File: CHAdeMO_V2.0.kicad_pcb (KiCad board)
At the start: 4 copper layers, 100 x 107.7 mm, 128 parts, among them IC1 ISO1050DUBR, IC2 ISO1050DUBR, IC3 ATSAM3X8CA-CU, J1 UJ2-BV-1-TH, J2 5810132011, J3 39-28-8020, J4 B2B-PH-K-S(LF)(SN), K1 V23086C1001A403-EV-BLBOX, Q1 IRLML0060TRPBF, Q2 IRLML0060TRPBF, Q3 IRLML0060TRPBF, Q4 IRLML0060TRPBF, Q5 DMP4065SQ-7, U1 M24M02-DRMN6TP, U3 VOM617A-4T, U4 VOM617A-4T, U5 VOM617A-4T, U6 VOM617A-4T, U7 VOM617A-4T, Y1 CRYSTAL 12MHZ, Y2 Crystal 32.768kHz

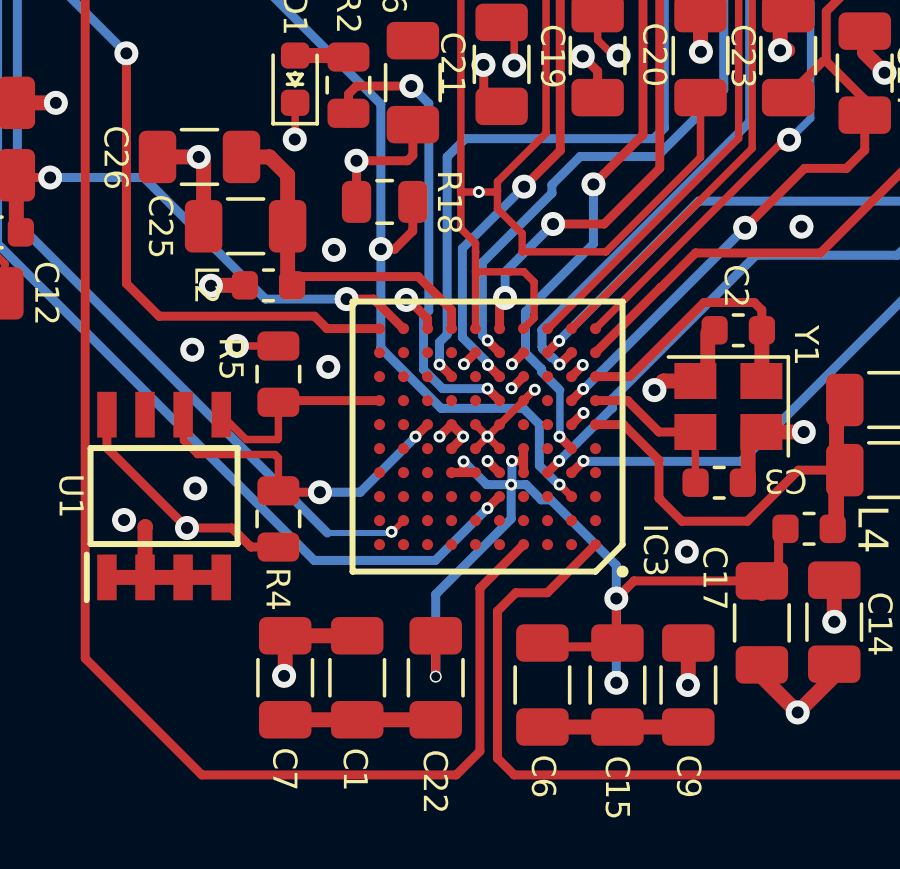
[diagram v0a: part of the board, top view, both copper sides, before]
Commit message: 2.0.3 Ball
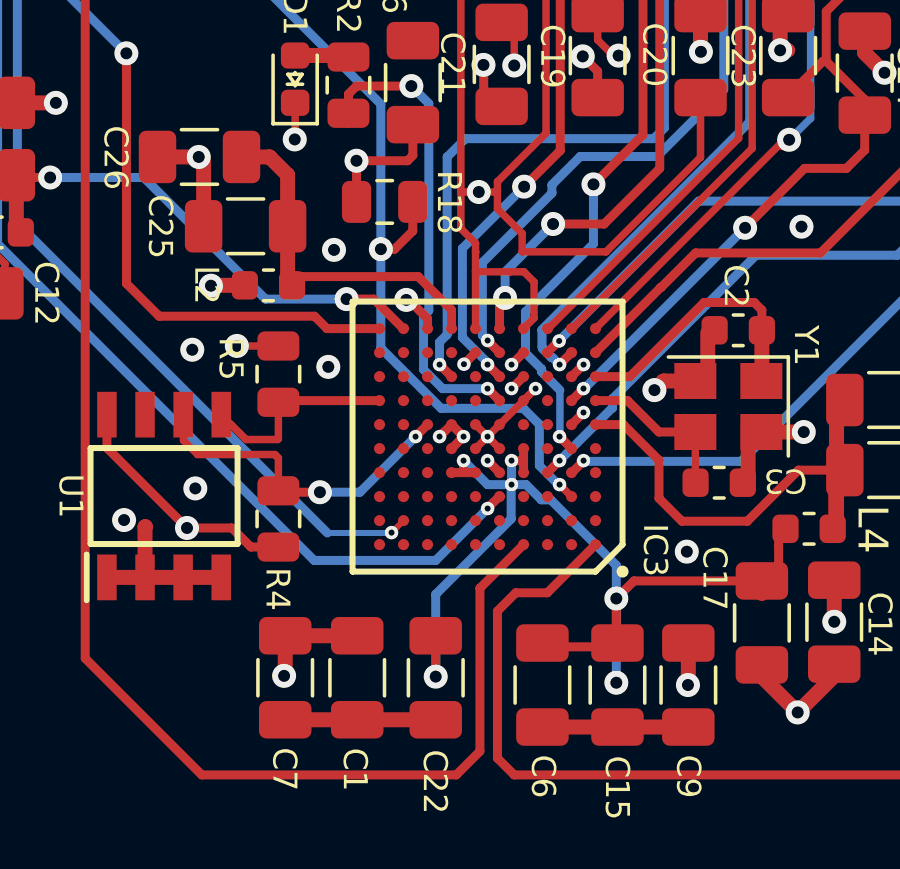
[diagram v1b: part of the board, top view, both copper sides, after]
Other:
- rule via_min_size: 0.4 -> 0.45
